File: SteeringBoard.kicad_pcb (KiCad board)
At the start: 2 copper layers, 59 x 26 mm, 76 parts, among them J1 SWD, J10 Conn_01x01_Pin, J11 Conn_01x01_Pin, J12 Conn_01x01_Pin, J13 Conn_01x01_Pin, J14 Conn_01x01_Pin, J15 Conn_01x01_Pin, J16 Conn_01x02_Pin, J17 Conn_01x01_Pin, J2 Conn_01x01_Pin, J3 Conn_01x01_Pin, J4 Conn_01x01_Pin, J5 Conn_01x01_Pin, J6 Conn_01x01_Pin, J7 Conn_01x01_Pin, J8 Conn_01x01_Pin, J9 Conn_01x01_Pin, SW1 Reset, U1 STM32L431CBTx, U2 ISO1044BD, U3 CDSOT23-T24CAN, U4 TPS562231DRLR, U5 RO-123.3S

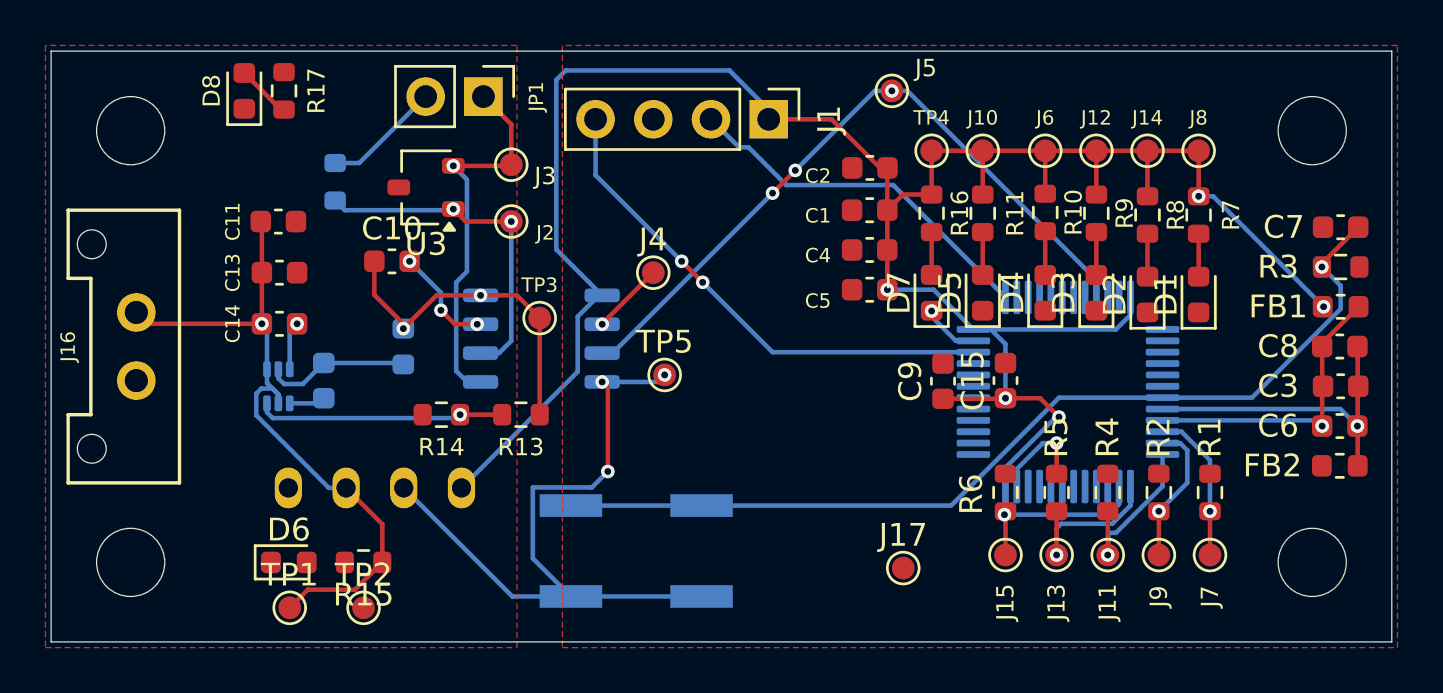
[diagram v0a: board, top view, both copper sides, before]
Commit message: board update
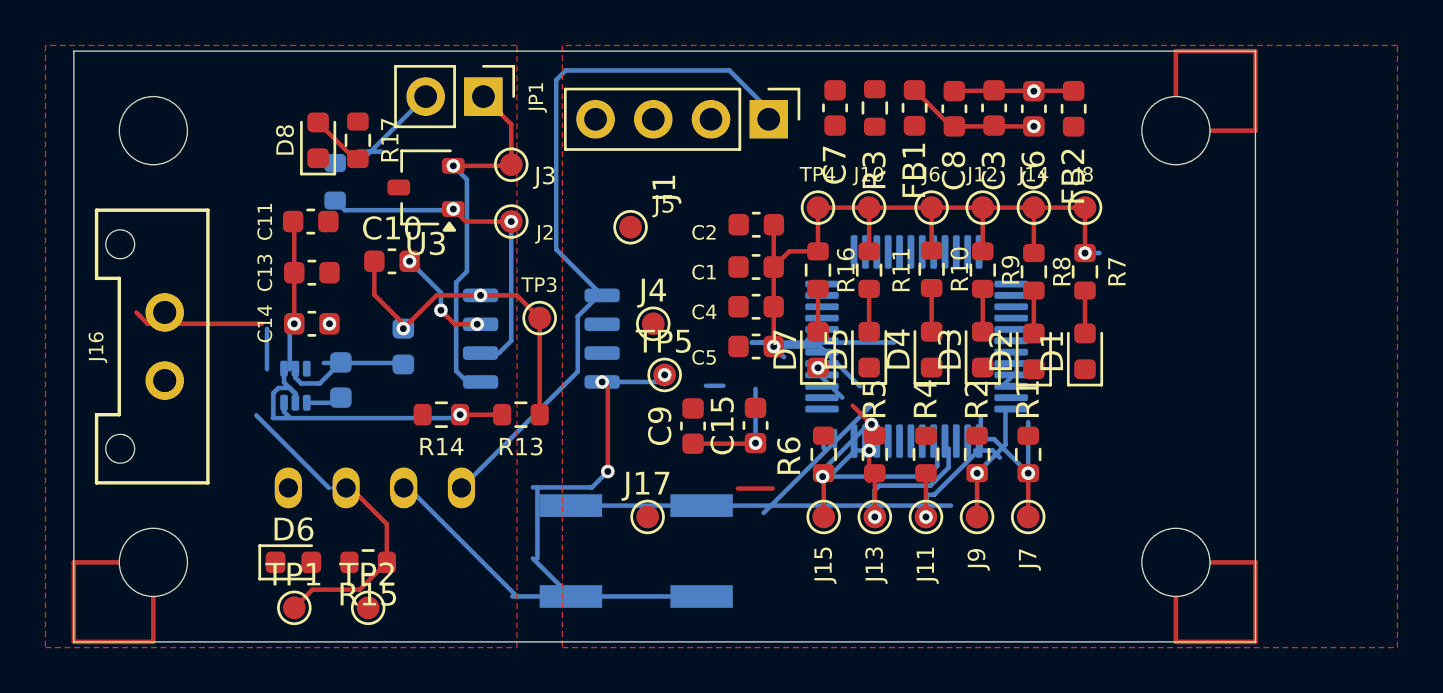
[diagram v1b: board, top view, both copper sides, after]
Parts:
- moved C7 22.9 mm to (155.8, 84.5), turned to -90 degrees
- moved R3 21.7 mm to (157.5, 84.5), turned to -90 degrees
- moved FB1 20.7 mm to (159.2, 84.5), turned to 90 degrees
- moved C8 19.9 mm to (161.0, 84.5), turned to 90 degrees
- moved FB2 19.6 mm to (166.2, 84.5), turned to 90 degrees
- moved C3 19.6 mm to (162.8, 84.5), turned to 90 degrees
- moved C6 19.4 mm to (164.5, 84.5), turned to 90 degrees
- moved J5 13.0 mm to (146.8, 89.8)
- moved J17 11.5 mm to (147.5, 102.5)
- moved C15 11.2 mm to (152.2, 98.5)
- moved C9 11.2 mm to (149.5, 98.5)
- moved J11 8.17 mm to (159.8, 102.5)
- moved J13 8.17 mm to (157.5, 102.5)
- moved J15 8.17 mm to (155.2, 102.5)
- moved J7 8.17 mm to (164.2, 102.5)
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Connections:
- J17 pad 1: /12V_Ext -> +12V
- R3 pad 1: VDD -> +3.3V
- U1 pad 8: GNDA -> unconnected-(U1-VSSA-Pad8)
- U1 pad 9: VDDA -> unconnected-(U1-VDDA-Pad9)
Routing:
- net /CAN_RX: track 30.7 -> 0.00 mm, vias 3 -> 0
- net /SWDIO: track 22.3 -> 0.00 mm, vias 2 -> 0
- net /NRST: track 42.1 -> 23.6 mm, vias 1 -> 0
- net /SWCLK: track 16.2 -> 0.00 mm
- net +3.3V: track 102.7 -> 89.6 mm, vias 5 -> 4
- net GNDA: track 14.1 -> 5.26 mm
- net VDDA: track 13.0 -> 6.27 mm
- net /CAN_TX: track 3.20 -> 0.00 mm, vias 1 -> 0
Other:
- board size 59 x 26 mm -> 52 x 26 mm
